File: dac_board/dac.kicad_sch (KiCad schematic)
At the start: 15 parts, among them IC1 ES9039Q2M, IC2 ES9312Q

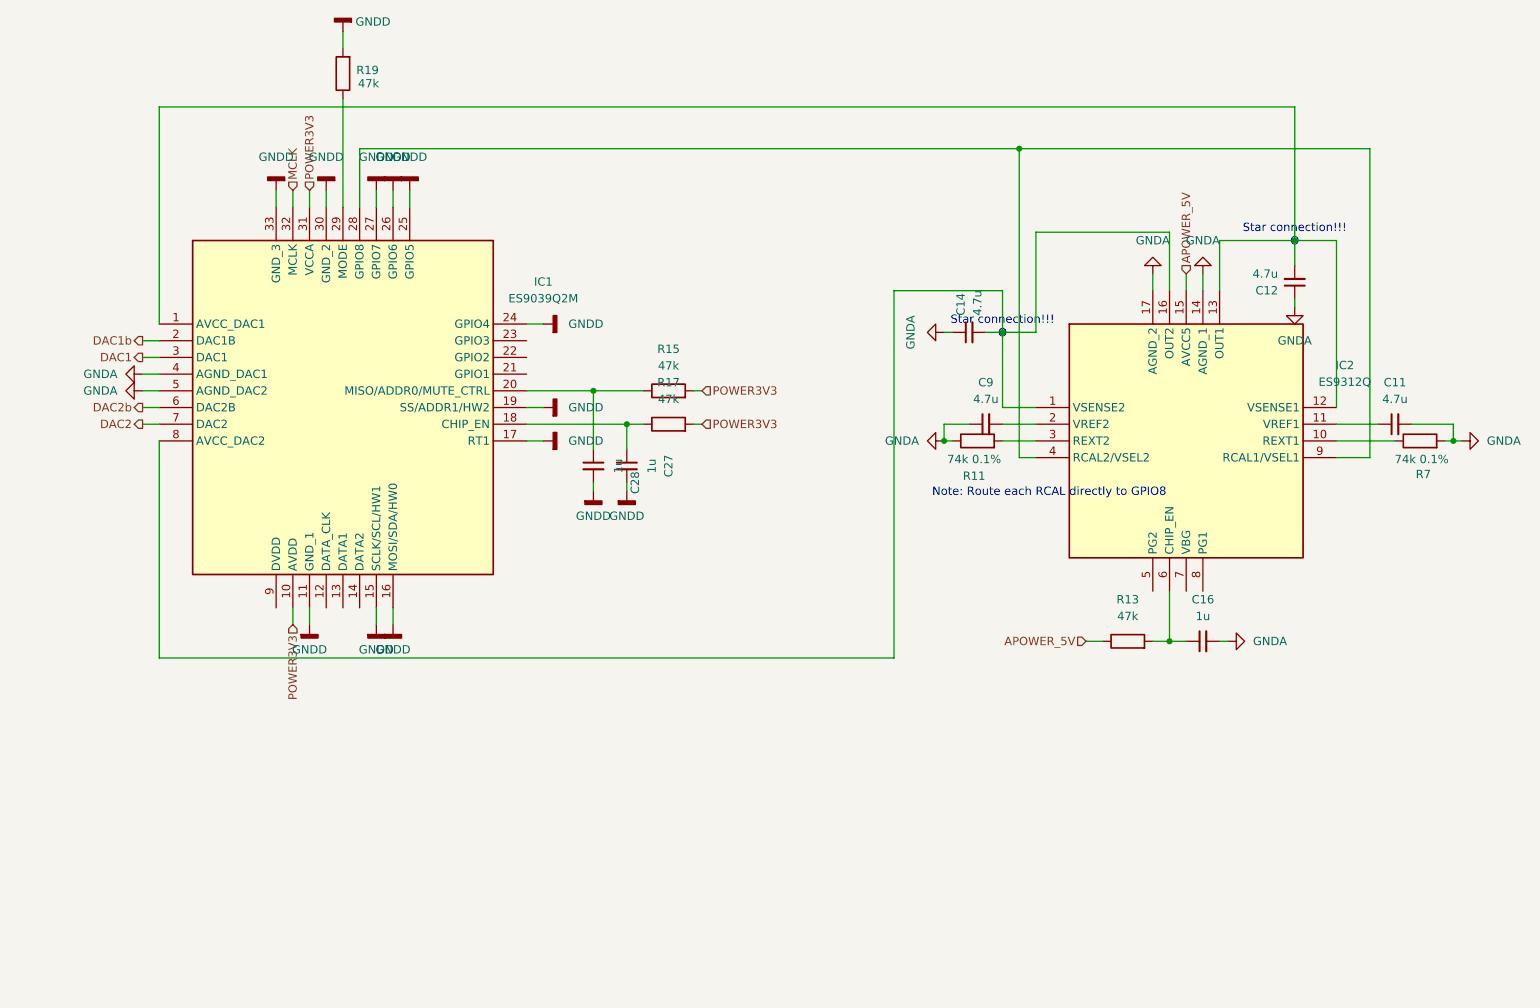
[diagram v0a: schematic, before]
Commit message: More updates, finished DAC block
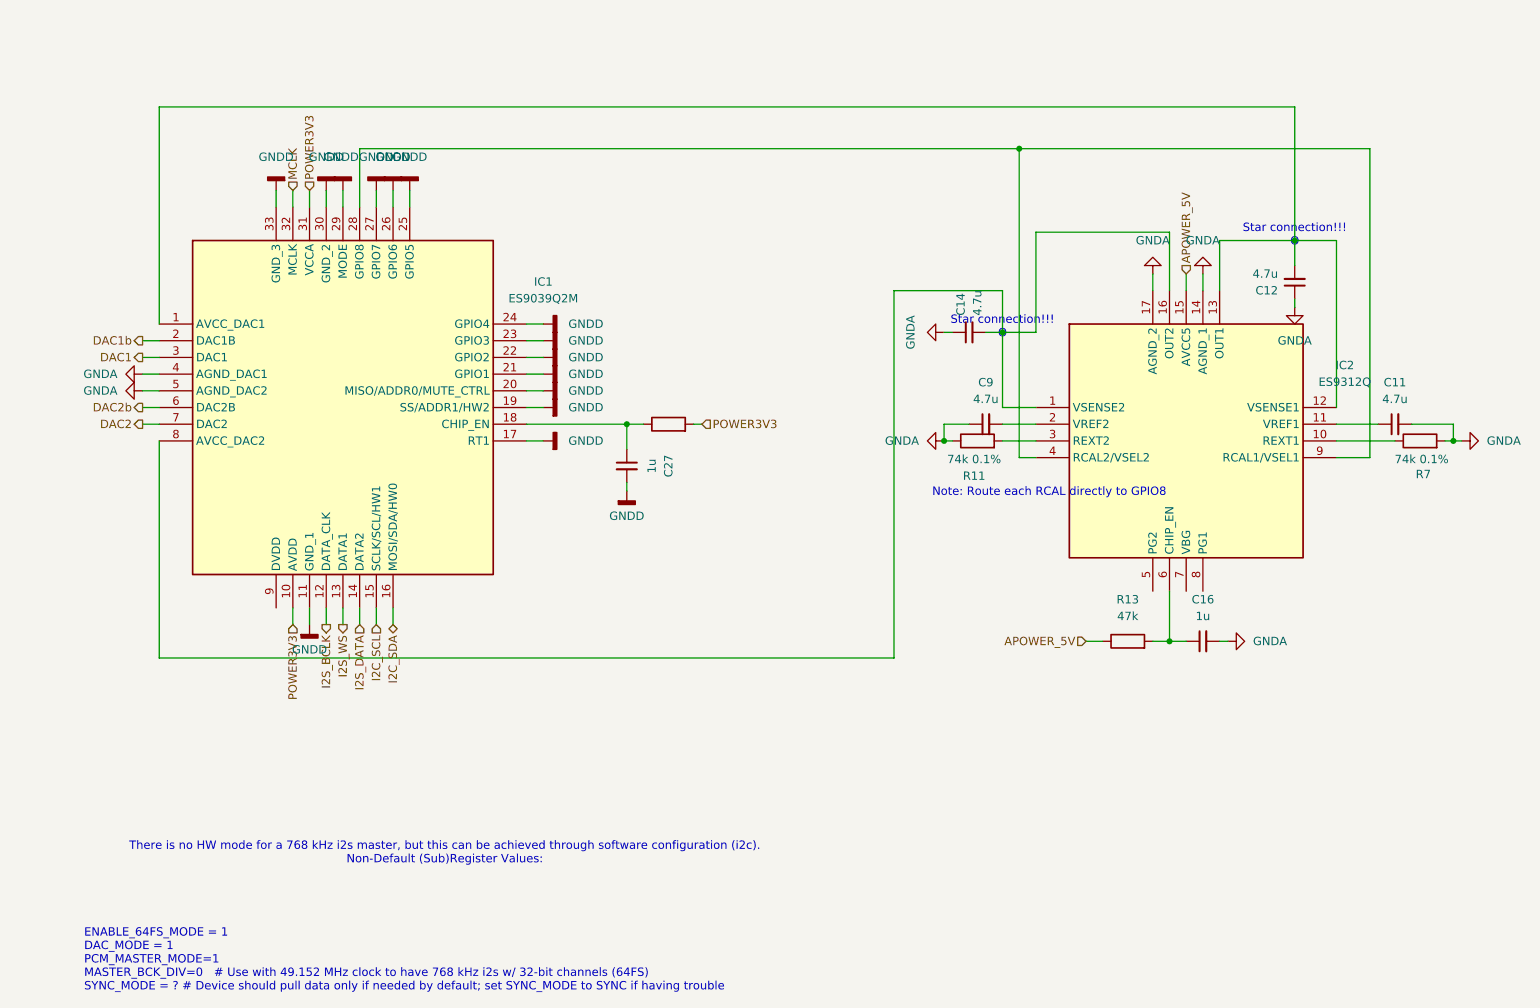
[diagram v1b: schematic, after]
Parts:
- removed C28: 1u, symbol Device:C_Small
- removed R15, R19: 47k, symbol Device:R
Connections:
- net GNDD: now also IC1.20 (MISO/ADDR0/MUTE_CTRL), IC1.21 (GPIO1), IC1.22 (GPIO2), IC1.23 (GPIO3), IC1.29 (MODE); no longer IC1.15 (SCLK/SCL/HW1), IC1.16 (MOSI/SDA/HW0)
- net I2S_BCLK: now reaches IC1.12 (DATA_CLK)
- net I2S_WS: now reaches IC1.13 (DATA1)
- net I2S_DATA: now reaches IC1.14 (DATA2)
- new net I2C_SCL: IC1.15 (SCLK/SCL/HW1)
- new net I2C_SDA: IC1.16 (MOSI/SDA/HW0)
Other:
- note added: "ENABLE_64FS_MODE = 1 r DAC_MODE = 1 r PCM_MASTER_MODE=1 r MASTER_BCK_DIV=0 # Use with 49.152 MHz clock to have 768 kHz i2s w/ 32-bit channels (64FS)r SYNC_MODE = ? # Device should pull data only if needed by default; set SYNC_MODE to SYNC if having trouble"
- note added: "There is no HW mode for a 768 kHz i2s master, but this can be achieved through software configuration (i2c). Non-Default (Sub)Register Values:"
- title: (none) -> DAC and DAC Power
